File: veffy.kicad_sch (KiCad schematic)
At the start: 109 parts, among them J1 SWD, J2 Conn_Coaxial, Q1 2N7002, Q2 BFR93A, Q3 2N7002, Q4 BFR93AE6327HTSA1, SW1 SW_Push, U1 ATSAMD21G18A-A, U2 ADF4112BCPZ, U3 SA612AN/01_112, U4 MC3361, U5 LM386, U6 LM358_DFN, U7 AD9834, U8 QPA9510, Y2 TCXO-14

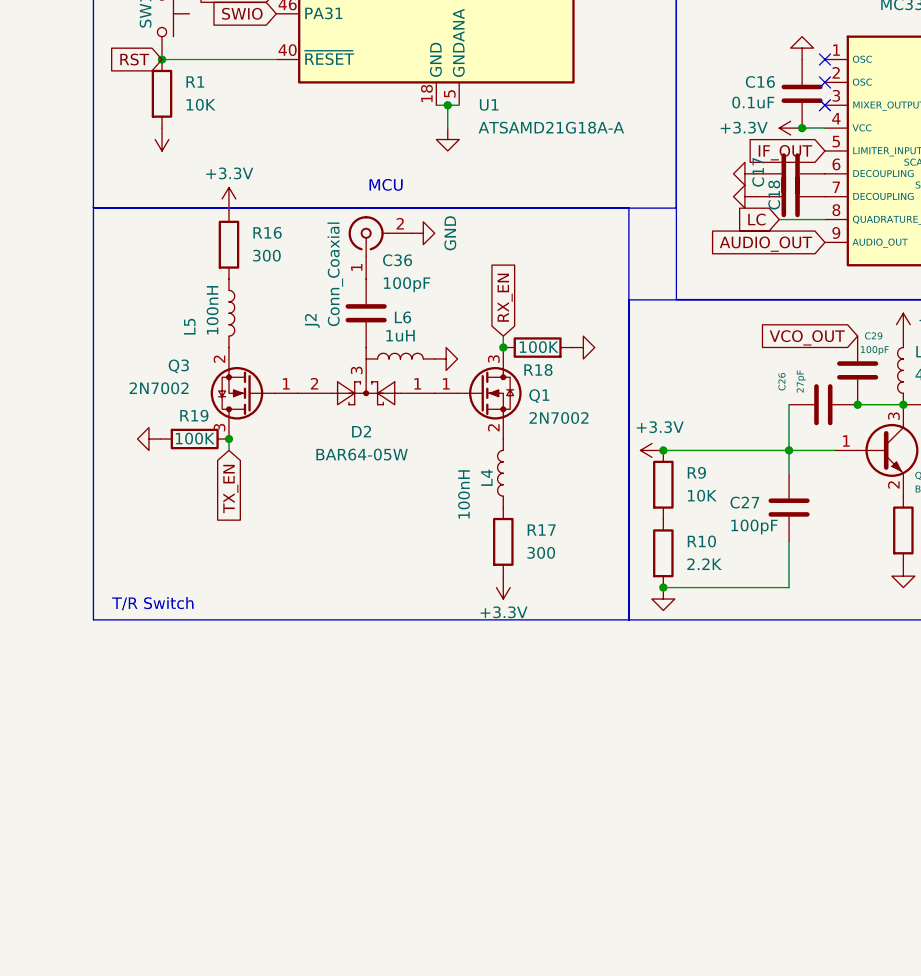
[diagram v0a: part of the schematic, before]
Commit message: rx pre-selector done
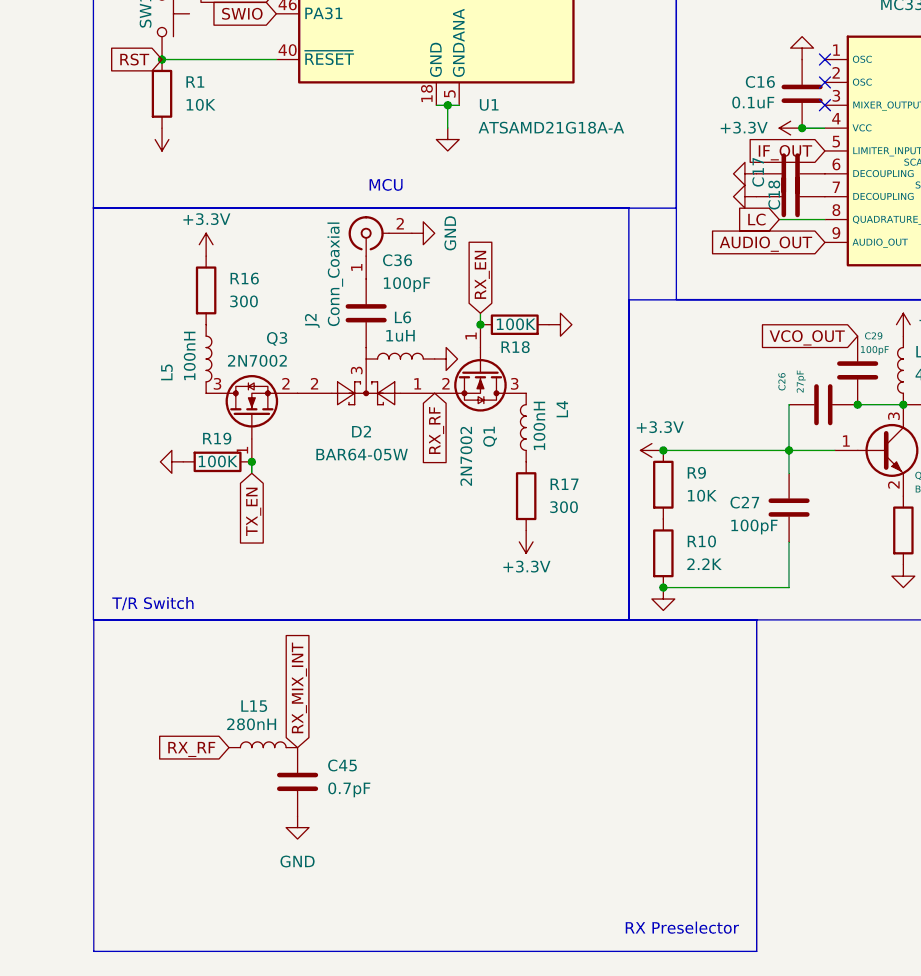
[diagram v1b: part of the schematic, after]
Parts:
- added C45: 0.7pF, symbol Device:C
- added L15: 280nH, Inductor_SMD:L_0603_1608Metric, symbol Device:L
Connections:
- net GND: now also C45.2
- net RX_EN: now also Q1.1 (G); no longer Q1.3 (D)
- net RX_MIX_INT: now also C45.1, L15.2
- net TX_EN: now also Q3.1 (G); no longer Q3.3 (D)
- net RX_RF: now reaches D2.1
- net RX_RF: now also Q1.2 (S), L15.1; no longer Q1.1 (G)
- net at L4.2: now also Q1.3 (D); no longer Q1.2 (S)
- net at D2.2: now also Q3.2 (S); no longer Q3.1 (G)
- net at L5.2: now also Q3.3 (D); no longer Q3.2 (S)
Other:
- note added: "RX Preselector"
- moved on the sheet: L4, L5, Q1, Q3, R16, R17, R18, R19
